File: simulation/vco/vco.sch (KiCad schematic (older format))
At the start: 8 parts, among them U1 LM324

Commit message: fixed that shit
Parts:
- removed R42: 100k, symbol Device:R
- removed R5, R6: 10k, symbol Device:R
- added R9001: 1T, symbol Device:R
- U1: Spice_Node_Sequence 1 2 4 5 3 -> 1,2,4,5,3
- V2: value 10 -> 1
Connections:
- net labels added: GNDREF, VCC, VEE, V_control
- net labels removed: +5V, -5V, GND
- wire segments 29 -> 31
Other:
- note added: ".tran 1m 1"
- note added: "Control\nvoltage"
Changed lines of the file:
@@
 Comment4 ""
 $EndDescr
-Wire Wire Line
-	2250 1400 2350 1400
 $Comp
 L pspice:OPAMP U1
@@
 F 5 "LM324" H 1950 1400 50  0001 C CNN "Spice_Model"
 F 6 "Y" H 1950 1400 50  0001 C CNN "Spice_Netlist_Enabled"
-F 7 "1 2 4 5 3" H 1950 1400 50  0001 C CNN "Spice_Node_Sequence"
-F 8 "LM324.ti.lib" H 1950 1400 50  0001 C CNN "Spice_Lib_File"
+F 7 "LM324.ti.lib" H 1950 1400 50  0001 C CNN "Spice_Lib_File"
+F 8 "1,2,4,5,3" H 1950 1400 50  0001 C CNN "Spice_Node_Sequence"
 	1    1950 1400
-	1    0    0    -1
-$EndComp
-Wire Wire Line
-	2350 1750 1650 1750
-Wire Wire Line
-	1650 1750 1650 1500
-Wire Wire Line
-	2350 1400 2350 1750
-$Comp
-L power:+5V #PWR?
-U 1 1 5CF04190
-P 1450 800
-F 0 "#PWR?" H 1450 650 50  0001 C CNN
-F 1 "+5V" H 1465 973 50  0000 C CNN
-F 2 "" H 1450 800 50  0001 C CNN
-F 3 "" H 1450 800 50  0001 C CNN
-	1    1450 800
 	1    0    0    -1
 $EndComp
@@
 U 1 1 5CF0529A
 P 1450 1550
-F 0 "R2" H 1300 1600 50  0000 L CNN
+F 0 "R2" H 1300 1500 50  0000 L CNN
 F 1 "100k" V 1450 1450 50  0000 L CNN
 F 2 "" V 1380 1550 50  0001 C CNN
@@
 Wire Wire Line
 	1450 1300 1450 1400
-$Comp
-L power:-5V #PWR?
-U 1 1 5CF05C0C
-P 1450 1900
-F 0 "#PWR?" H 1450 2000 50  0001 C CNN
-F 1 "-5V" H 1465 2073 50  0000 C CNN
-F 2 "" H 1450 1900 50  0001 C CNN
-F 3 "" H 1450 1900 50  0001 C CNN
-	1    1450 1900
-	-1   0    0    1
-$EndComp
 Wire Wire Line
 	1850 1850 1850 1700
@@
 Wire Wire Line
 	1450 850  1450 900
-$Comp
-L power:GND #PWR?
-U 1 1 5CF06DC5
-P 2550 1550
-F 0 "#PWR?" H 2550 1300 50  0001 C CNN
-F 1 "GND" H 2555 1377 50  0000 C CNN
-F 2 "" H 2550 1550 50  0001 C CNN
-F 3 "" H 2550 1550 50  0001 C CNN
-	1    2550 1550
-	1    0    0    -1
-$EndComp
 Wire Wire Line
 	2550 1550 2550 1400
-Wire Wire Line
-	2550 1400 2350 1400
-Connection ~ 2350 1400
 Text Notes 2000 1100 0    50   ~ 0
 Rail splitter:\nVirtual Ground
@@
 Connection ~ 1450 1850
 Wire Wire Line
+	1850 1850 1450 1850
+Text Notes 550  600  0    50   ~ 0
+.tran 1m 1
+Wire Wire Line
+	1600 1750 1600 1500
+Wire Wire Line
+	1600 1500 1650 1500
+Wire Wire Line
+	1600 1750 2350 1750
+$Comp
+L power:VCC #PWR?
+U 1 1 5CF0E364
+P 1450 800
+F 0 "#PWR?" H 1450 650 50  0001 C CNN
+F 1 "VCC" H 1467 973 50  0000 C CNN
+F 2 "" H 1450 800 50  0001 C CNN
+F 3 "" H 1450 800 50  0001 C CNN
+	1    1450 800
+	1    0    0    -1
+$EndComp
+$Comp
+L power:VEE #PWR?
+U 1 1 5CF0FCB5
+P 1450 1900
+F 0 "#PWR?" H 1450 1750 50  0001 C CNN
+F 1 "VEE" H 1468 2073 50  0000 C CNN
+F 2 "" H 1450 1900 50  0001 C CNN
+F 3 "" H 1450 1900 50  0001 C CNN
+	1    1450 1900
+	-1   0    0    1
+$EndComp
+Wire Wire Line
 	1450 1850 1450 1900
 Wire Wire Line
-	1850 1850 1450 1850
+	2250 1400 2350 1400
+Wire Wire Line
+	2350 1400 2350 1750
+Connection ~ 2350 1400
+Wire Wire Line
+	2350 1400 2550 1400
 $Comp
 L pspice:0 #GND?
-U 1 1 5CF017AB
-P 2850 850
-F 0 "#GND?" H 2850 750 50  0001 C CNN
-F 1 "0" H 2850 750 50  0000 C CNN
-F 2 "" H 2850 850 50  0001 C CNN
-F 3 "~" H 2850 850 50  0001 C CNN
-	1    2850 850
-	1    0    0    -1
-$EndComp
-$Comp
-L power:GND #PWR?
-U 1 1 5CF026EA
-P 2700 800
-F 0 "#PWR?" H 2700 550 50  0001 C CNN
-F 1 "GND" H 2705 627 50  0000 C CNN
-F 2 "" H 2700 800 50  0001 C CNN
-F 3 "" H 2700 800 50  0001 C CNN
-	1    2700 800
-	1    0    0    -1
-$EndComp
-Wire Wire Line
-	2850 850  2850 700
-Wire Wire Line
-	2850 700  2700 700
-Wire Wire Line
-	2700 700  2700 800
-$Comp
-L power:+5V #PWR?
-U 1 1 5CF04FF6
-P 1700 2450
-F 0 "#PWR?" H 1700 2300 50  0001 C CNN
-F 1 "+5V" H 1715 2623 50  0000 C CNN
-F 2 "" H 1700 2450 50  0001 C CNN
-F 3 "" H 1700 2450 50  0001 C CNN
-	1    1700 2450
-	1    0    0    -1
-$EndComp
-$Comp
-L power:GND #PWR?
-U 1 1 5CF05313
-P 1700 2750
-F 0 "#PWR?" H 1700 2500 50  0001 C CNN
-F 1 "GND" H 1705 2577 50  0000 C CNN
-F 2 "" H 1700 2750 50  0001 C CNN
-F 3 "" H 1700 2750 50  0001 C CNN
-	1    1700 2750
-	1    0    0    -1
-$EndComp
-$Comp
-L Device:R R5
-U 1 1 5CF0559F
-P 1700 2600
-F 0 "R5" H 1550 2650 50  0000 L CNN
-F 1 "10k" V 1700 2500 50  0000 L CNN
-F 2 "" V 1630 2600 50  0001 C CNN
-F 3 "~" H 1700 2600 50  0001 C CNN
-	1    1700 2600
-	1    0    0    -1
-$EndComp
-$Comp
-L power:GND #PWR?
-U 1 1 5CF06A87
-P 2100 2750
-F 0 "#PWR?" H 2100 2500 50  0001 C CNN
-F 1 "GND" H 2105 2577 50  0000 C CNN
-F 2 "" H 2100 2750 50  0001 C CNN
-F 3 "" H 2100 2750 50  0001 C CNN
-	1    2100 2750
-	1    0    0    -1
-$EndComp
-$Comp
-L Device:R R6
-U 1 1 5CF06A91
-P 2100 2600
-F 0 "R6" H 1950 2650 50  0000 L CNN
-F 1 "10k" V 2100 2500 50  0000 L CNN
-F 2 "" V 2030 2600 50  0001 C CNN
-F 3 "~" H 2100 2600 50  0001 C CNN
-	1    2100 2600
-	1    0    0    -1
-$EndComp
-$Comp
-L power:-5V #PWR?
-U 1 1 5CF07790
-P 2100 2450
-F 0 "#PWR?" H 2100 2550 50  0001 C CNN
-F 1 "-5V" H 2115 2623 50  0000 C CNN
-F 2 "" H 2100 2450 50  0001 C CNN
-F 3 "" H 2100 2450 50  0001 C CNN
-	1    2100 2450
-	1    0    0    -1
-$EndComp
-$Comp
-L power:GND #PWR?
-U 1 1 5CF0805C
-P 3600 2100
-F 0 "#PWR?" H 3600 1850 50  0001 C CNN
-F 1 "GND" H 3605 1927 50  0000 C CNN
-F 2 "" H 3600 2100 50  0001 C CNN
-F 3 "" H 3600 2100 50  0001 C CNN
-	1    3600 2100
+U 1 1 5CF02FCA
+P 1050 2000
+F 0 "#GND?" H 1050 1900 50  0001 C CNN
+F 1 "0" H 1000 2100 50  0000 C CNN
+F 2 "" H 1050 2000 50  0001 C CNN
+F 3 "~" H 1050 2000 50  0001 C CNN
+	1    1050 2000
+	1    0    0    -1
+$EndComp
+Connection ~ 1050 1850
+Wire Wire Line
+	1050 2000 1050 1850
+$Comp
+L power:GNDREF #PWR?
+U 1 1 5CF0644C
+P 2550 1550
+F 0 "#PWR?" H 2550 1300 50  0001 C CNN
+F 1 "GNDREF" H 2555 1377 50  0000 C CNN
+F 2 "" H 2550 1550 50  0001 C CNN
+F 3 "" H 2550 1550 50  0001 C CNN
+	1    2550 1550
 	1    0    0    -1
 $EndComp
 $Comp
 L pspice:VSOURCE V2
-U 1 1 5CF0849D
-P 3600 1750
-F 0 "V2" H 3828 1796 50  0000 L CNN
-F 1 "10" H 3828 1705 50  0000 L CNN
-F 2 "" H 3600 1750 50  0001 C CNN
-F 3 "~" H 3600 1750 50  0001 C CNN
-	1    3600 1750
-	1    0    0    -1
-$EndComp
-Wire Wire Line
-	3600 2050 3600 2100
-Wire Wire Line
-	3600 1350 3600 1450
-Wire Wire Line
-	3600 1050 3950 1050
-Wire Wire Line
-	3950 1050 3950 2100
-Wire Wire Line
-	3950 2100 3600 2100
-Connection ~ 3600 2100
-$Comp
-L Device:R R42
-U 1 1 5CF08CA9
-P 3600 1200
-F 0 "R42" H 3670 1246 50  0000 L CNN
-F 1 "100k" H 3670 1155 50  0000 L CNN
-F 2 "" V 3530 1200 50  0001 C CNN
-F 3 "~" H 3600 1200 50  0001 C CNN
-	1    3600 1200
-	1    0    0    -1
-$EndComp
+U 1 1 5CF0AB02
+P 3350 1450
+F 0 "V2" H 2950 1550 50  0000 L CNN
+F 1 "1" H 2950 1300 50  0000 L CNN
+F 2 "" H 3350 1450 50  0001 C CNN
+F 3 "~" H 3350 1450 50  0001 C CNN
+	1    3350 1450
+	1    0    0    -1
+$EndComp
+$Comp
+L power:GNDREF #PWR?
+U 1 1 5CF0AF65
+P 3350 1850
+F 0 "#PWR?" H 3350 1600 50  0001 C CNN
+F 1 "GNDREF" H 3355 1677 50  0000 C CNN
+F 2 "" H 3350 1850 50  0001 C CNN
+F 3 "" H 3350 1850 50  0001 C CNN
+	1    3350 1850
+	1    0    0    -1
+$EndComp
+Text GLabel 3350 1050 1    50   Input ~ 0
+V_control
+$Comp
+L Device:R R9001
+U 1 1 5CF0C88B
+P 3800 1450
+F 0 "R9001" H 3870 1496 50  0000 L CNN
+F 1 "1T" H 3870 1405 50  0000 L CNN
+F 2 "" V 3730 1450 50  0001 C CNN
+F 3 "~" H 3800 1450 50  0001 C CNN
+	1    3800 1450
+	1    0    0    -1
+$EndComp
+Wire Wire Line
+	3350 1150 3350 1100
+Wire Wire Line
+	3350 1100 3800 1100
+Wire Wire Line
+	3800 1100 3800 1300
+Connection ~ 3350 1100
+Wire Wire Line
+	3350 1100 3350 1050
+Wire Wire Line
+	3350 1850 3350 1800
+Wire Wire Line
+	3350 1800 3800 1800
+Wire Wire Line
+	3800 1800 3800 1600
+Connection ~ 3350 1800
+Wire Wire Line
+	3350 1800 3350 1750
+Text Notes 3500 950  0    50   ~ 0
+Control\nvoltage
 $EndSCHEMATC

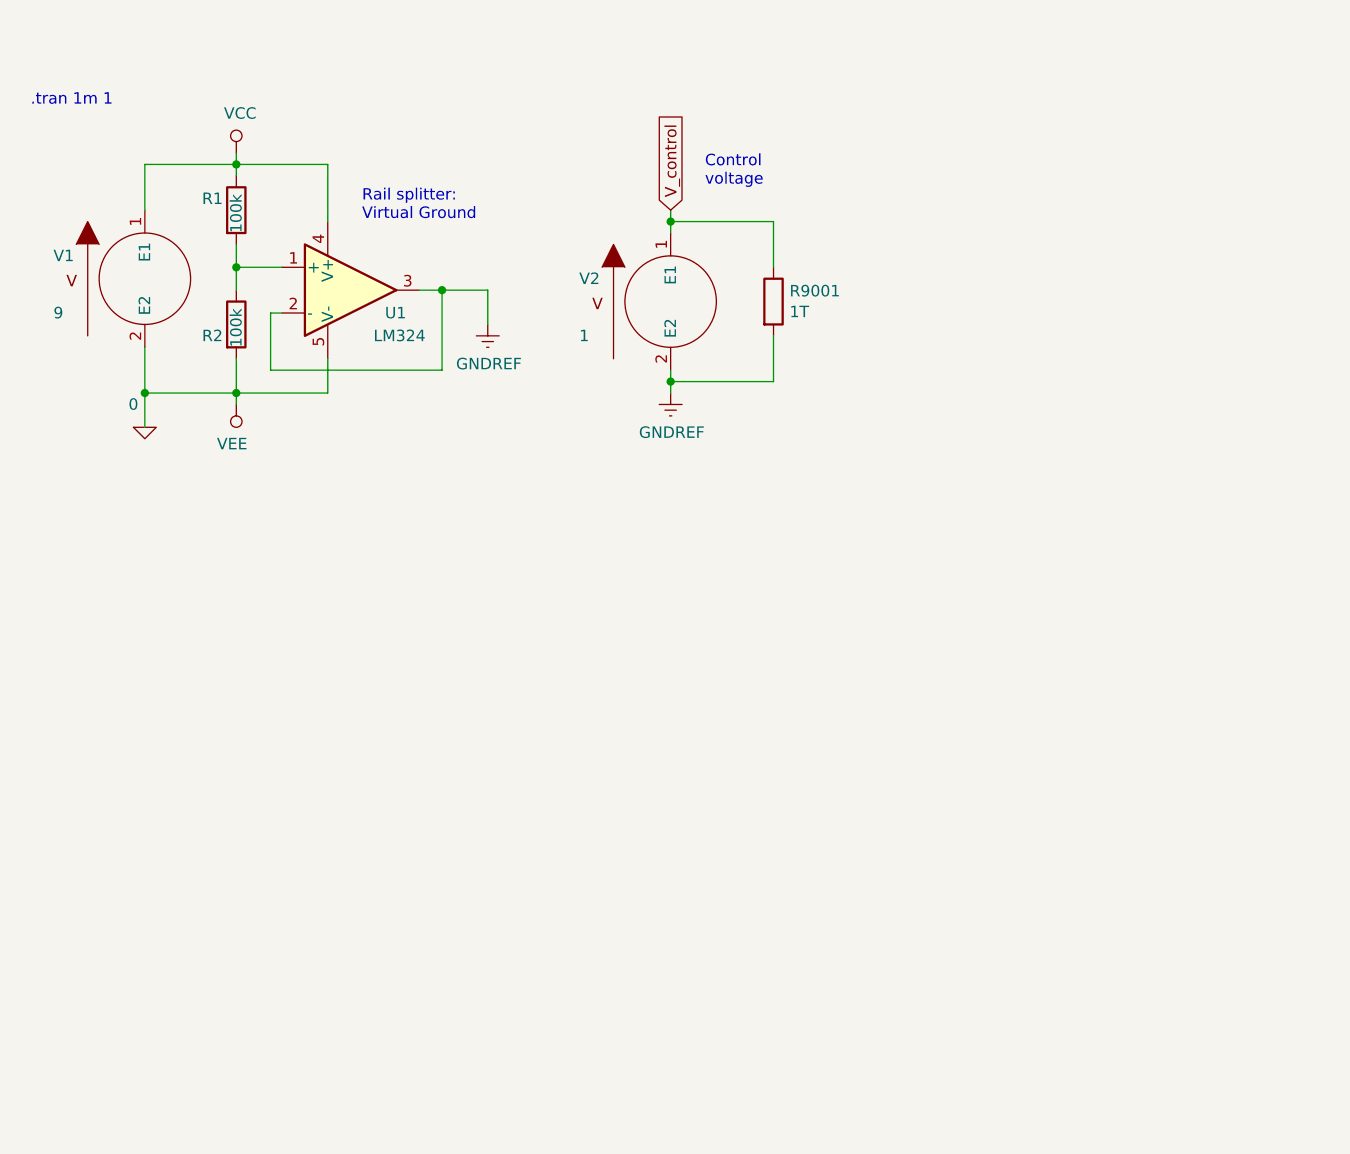
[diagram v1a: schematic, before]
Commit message: vco :)
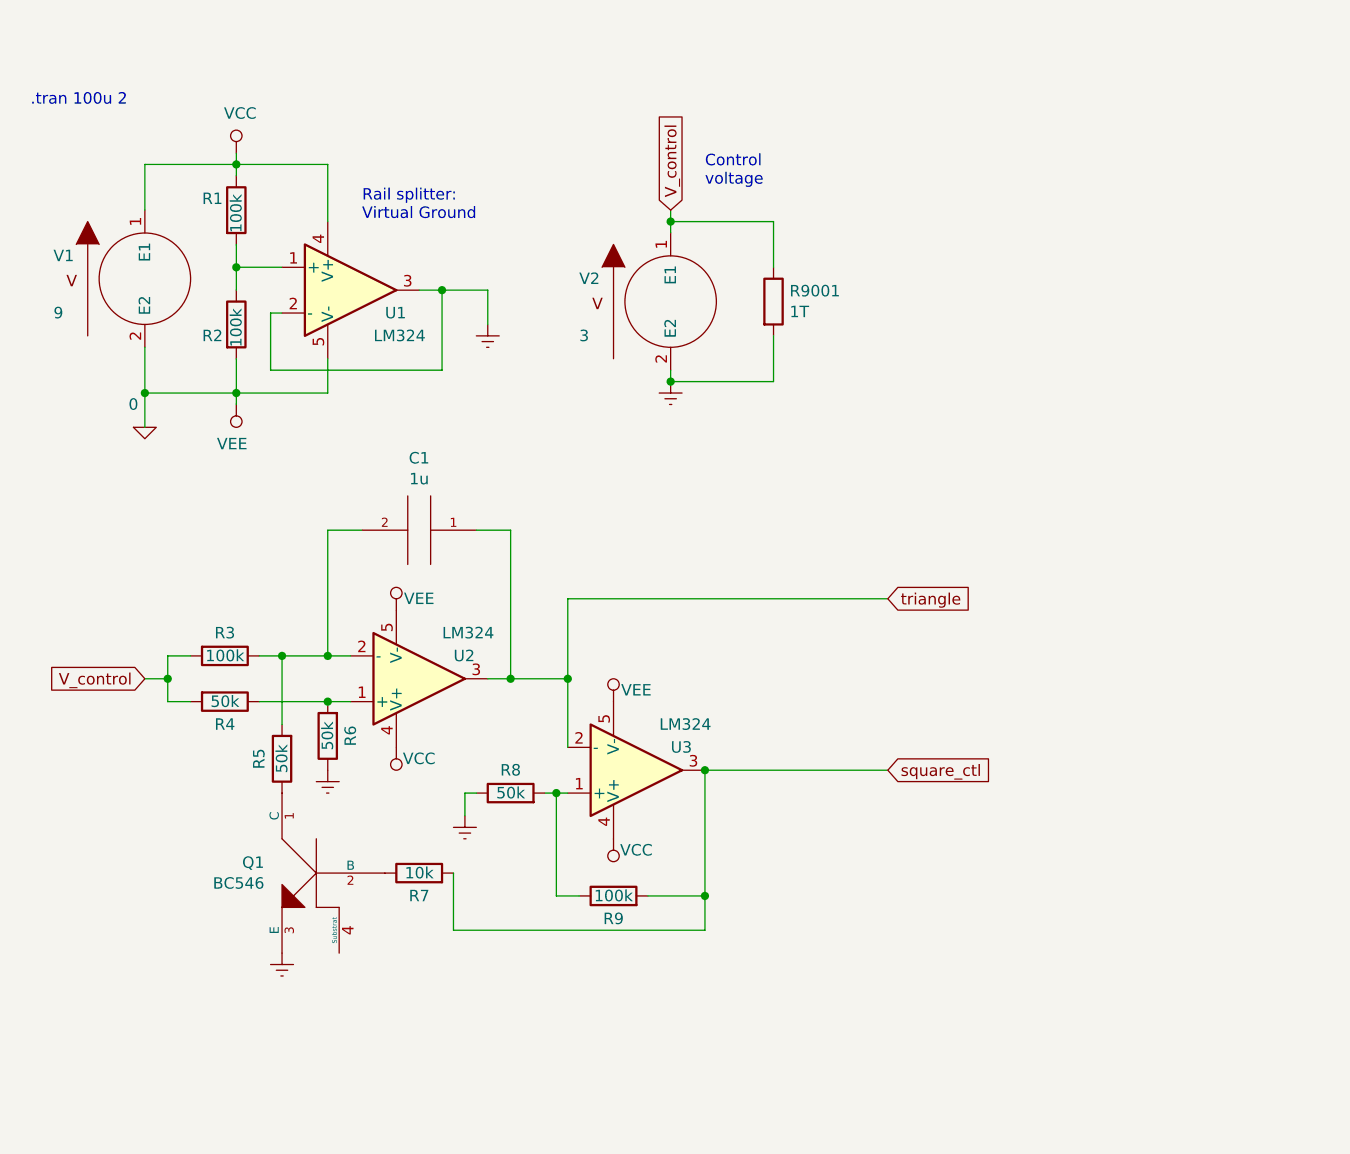
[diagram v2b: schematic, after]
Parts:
- added C1: 1u, symbol pspice:C
- added Q1: BC546, symbol pspice:QNPN
- added R3, R9: 100k, symbol Device:R
- added R4, R5, R6, R8: 50k, symbol Device:R
- added R7: 10k, symbol Device:R
- added U2, U3: LM324, symbol pspice:OPAMP
- V2: value 1 -> 3
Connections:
- net 0: now also U2.5 (V-), U3.5 (V-)
- net GNDREF: now also Q1.3 (E), R6.1, R8.1
- net VCC: now also U2.4 (V+), U3.4 (V+)
- net V_control: now also R3.2, R4.2
- new net: R4.1, R6.2, U2.1 (+)
- new net: C1.2, R3.1, R5.2, U2.2 (-)
- new net: Q1.1 (C), R5.1
- new net: Q1.2 (B), R7.1
- new net: R8.2, R9.1, U3.1 (+)
- new net square_ctl: R7.2, R9.2, U3.3
- new net triangle: C1.1, U2.3, U3.2 (-)
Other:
- note added: ".tran 100u 2"
- note removed: ".tran 1m 1"

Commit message: sawtooth broken?
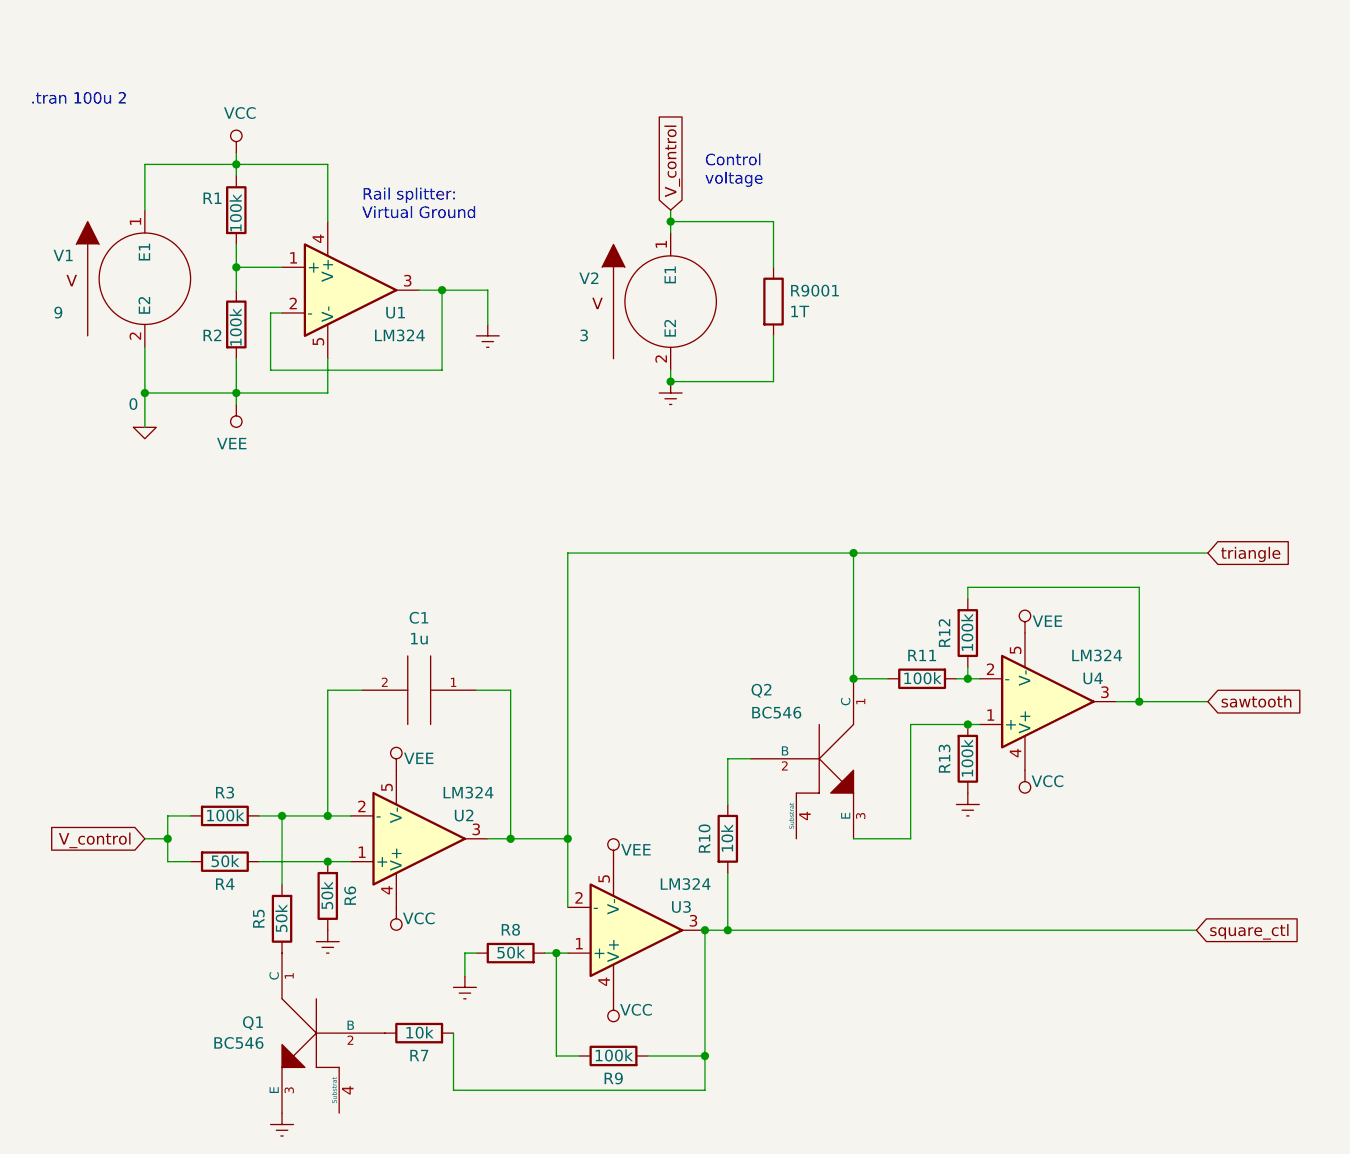
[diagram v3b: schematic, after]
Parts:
- added Q2: BC546, symbol pspice:QNPN
- added R10: 10k, symbol Device:R
- added R11, R12, R13: 100k, symbol Device:R
- added U4: LM324, symbol pspice:OPAMP
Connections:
- net 0: now also U4.5 (V-)
- net GNDREF: now also R13.1
- net VCC: now also U4.4 (V+)
- net square_ctl: now also R10.2
- net triangle: now also Q2.1 (C), R11.1
- new net: Q2.3 (E), R13.2, U4.1 (+)
- new net: R11.2, R12.1, U4.2 (-)
- new net: Q2.2 (B), R10.1
- new net sawtooth: R12.2, U4.3
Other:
- moved on the sheet: C1, Q1, R3, R4, R5, R6, R7, R8, R9, U2, U3
